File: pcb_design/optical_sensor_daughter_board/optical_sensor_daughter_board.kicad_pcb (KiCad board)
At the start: 2 copper layers, 22.9 x 44.5 mm, 2 parts, among them J1 Conn_02x06_Counter_Clockwise, U1 PMW3389

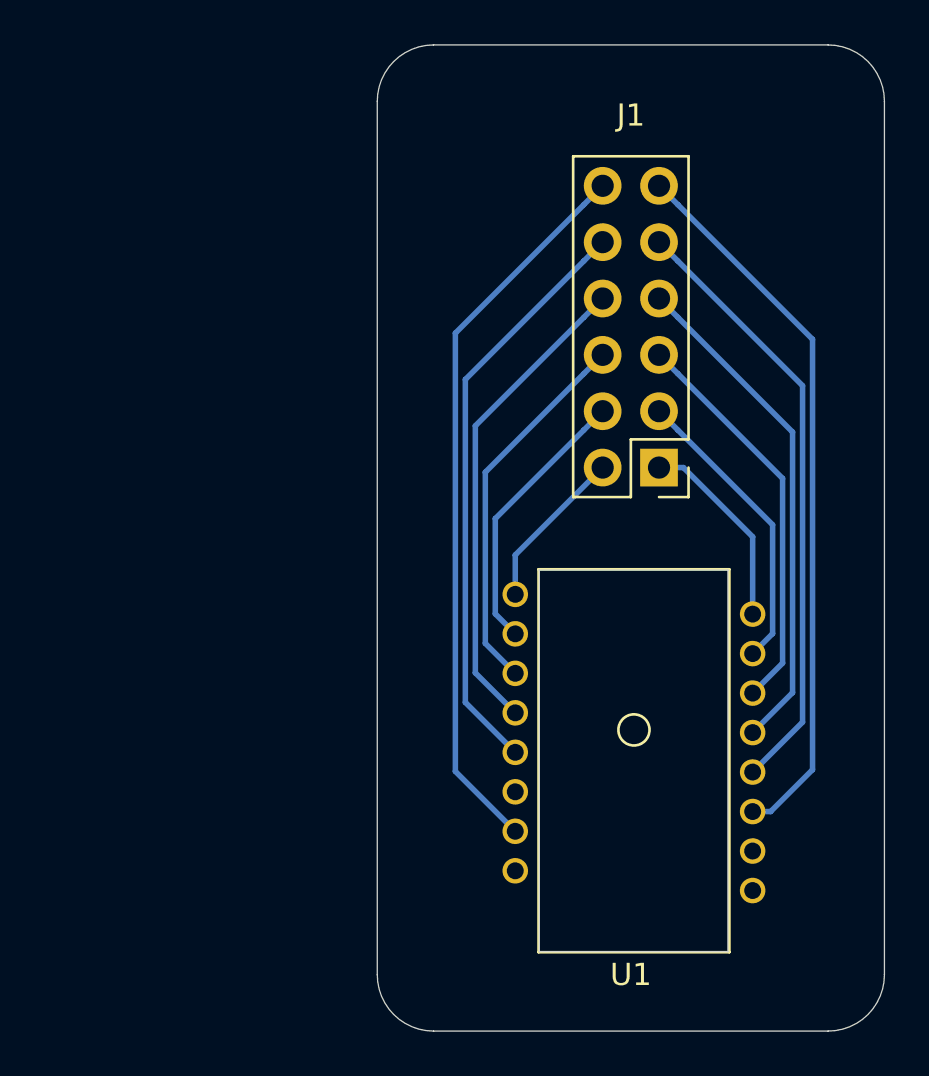
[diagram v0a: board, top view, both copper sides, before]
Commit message: WIP daughter board
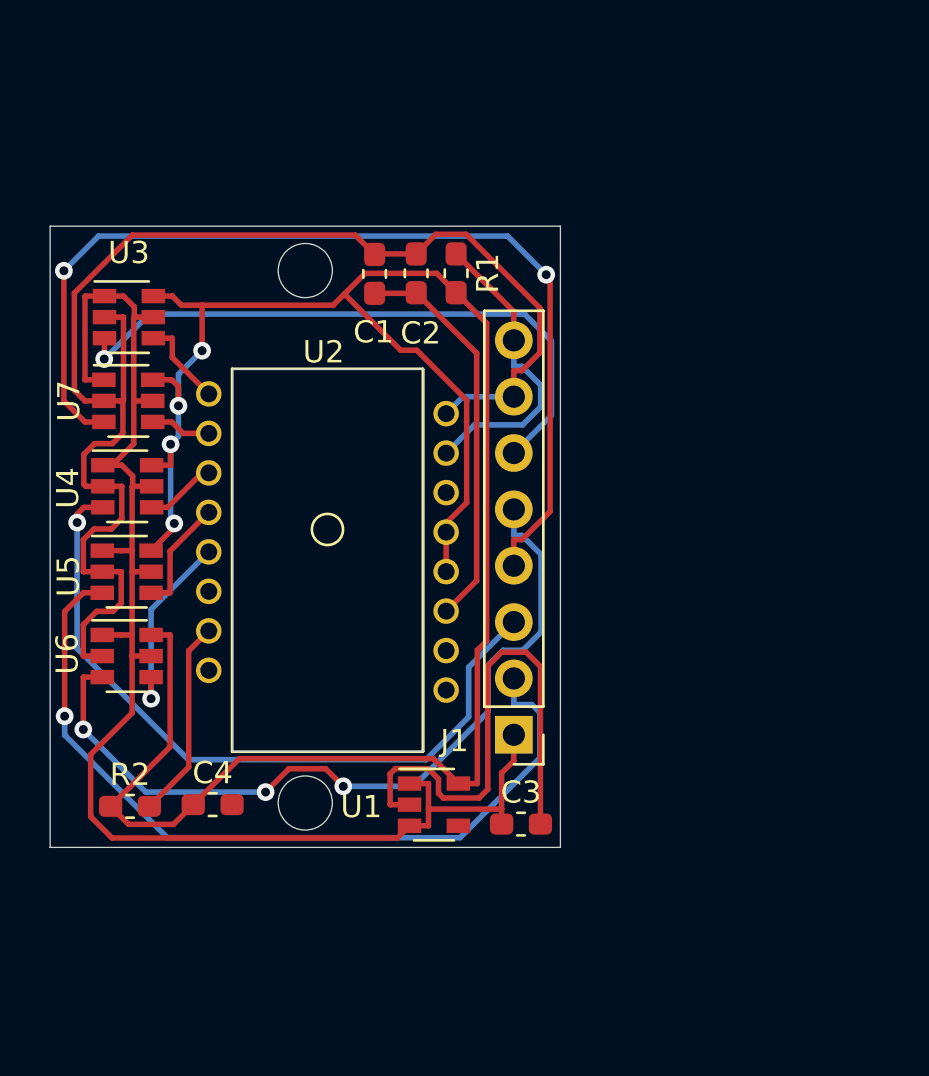
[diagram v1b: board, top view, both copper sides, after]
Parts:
- added C1: 0.1uF, Capacitor_SMD:C_0603_1608Metric_Pad1.05x0.95mm_HandSolder, F.Cu at (137.7, 85.2)
- added C2: 4.7uF, Capacitor_SMD:C_0603_1608Metric_Pad1.05x0.95mm_HandSolder, F.Cu at (139.6, 85.2)
- added C3: 1uF, Capacitor_SMD:C_0603_1608Metric_Pad1.05x0.95mm_HandSolder, F.Cu at (144.3, 110.0)
- added C4: 1uF, Capacitor_SMD:C_0603_1608Metric_Pad1.05x0.95mm_HandSolder, F.Cu at (130.4, 109.2)
- added R1: 10K, Resistor_SMD:R_0603_1608Metric_Pad1.05x0.95mm_HandSolder, F.Cu at (141.3, 85.2)
- added R2: 39, Resistor_SMD:R_0603_1608Metric_Pad1.05x0.95mm_HandSolder, F.Cu at (126.7, 109.2)
- added U2: PMW3360, pmw3389:PMW3389, F.Cu at (135.6, 96.8)
- added U3: SN74LVC1T45DBV, Package_TO_SOT_SMD:SOT-23-6, F.Cu at (126.6, 87.2)
- added U4: SN74LVC1T45DBV, Package_TO_SOT_SMD:SOT-23-6, F.Cu at (126.5, 94.8)
- added U5: SN74LVC1T45DBV, Package_TO_SOT_SMD:SOT-23-6, F.Cu at (126.5, 98.7)
- added U6: SN74LVC1T45DBV, Package_TO_SOT_SMD:SOT-23-6, F.Cu at (126.5, 102.5)
- added U7: SN74LVC1T45DBV, Package_TO_SOT_SMD:SOT-23-6, F.Cu at (126.6, 91.0)
- J1: value Conn_02x06_Counter_Clockwise -> Conn_01x08_Male; footprint Connector_PinHeader_2.54mm:PinHeader_2x06_P2.54mm_Vertical -> Connector_PinHeader_2.54mm:PinHeader_1x08_P2.54mm_Vertical
- U1: value PMW3389 -> TLV70019_SOT23-5; footprint pmw3389:PMW3389 -> Package_TO_SOT_SMD:SOT-23-5
- moved J1 13.7 mm to (143.9, 106.0)
- moved U1 9.62 mm to (140.3, 109.2)
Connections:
- J1 pad 1: GND -> VIN
- J1 pad 2: MOTION -> MISO_3.3V
- J1 pad 3: NRESET -> MOIS_3.3V
- J1 pad 4: SCLK -> SLCK_3.3V
- J1 pad 5: GPO -> SS_3.3V
- J1 pad 6: MOSI -> MOTION_3.3V
- J1 pad 7: VDDIO -> GND
- J1 pad 8: MISO -> RESET
- U1 pad 1: (no net) -> VIN
- U1 pad 2: (no net) -> Net-(C3-Pad2)
- U1 pad 3: VDCPIX -> VIN
- U1 pad 4: VDD -> (no net)
- U1 pad 5: VDDIO -> VDD
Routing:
- net VDD: track 27.5 -> 97.6 mm, vias 0 -> 4
- net VIN: track 0.00 -> 65.4 mm
- net GND: track 9.00 -> 62.9 mm
- net SLCK_3.3V: track 0.00 -> 45.3 mm, vias 0 -> 2
- net MISO_3.3V: track 0.00 -> 37.0 mm, vias 0 -> 1
- net SS_3.3V: track 0.00 -> 36.1 mm, vias 0 -> 3
- net MOIS_3.3V: track 0.00 -> 33.0 mm, vias 0 -> 1
- net LED_P: track 33.0 -> 0.00 mm
- net VDCPIX: track 32.7 -> 0.00 mm
- net MOTION_3.3V: track 0.00 -> 28.2 mm, vias 0 -> 1
- net NCS: track 26.5 -> 0.00 mm
- net Net-(C3-Pad2): track 0.00 -> 23.4 mm
- net VDDIO: track 22.8 -> 0.00 mm
- net GPO: track 18.1 -> 0.00 mm
- net Net-(C1-Pad2): track 0.00 -> 17.9 mm
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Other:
- board size 22.9 x 44.5 mm -> 23 x 28 mm
